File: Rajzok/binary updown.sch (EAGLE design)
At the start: 17 parts, among them Q1 TP0602N2, Q2 TP0602N2, Q3 SUP75N06-08, Q4 SUP75N06-08

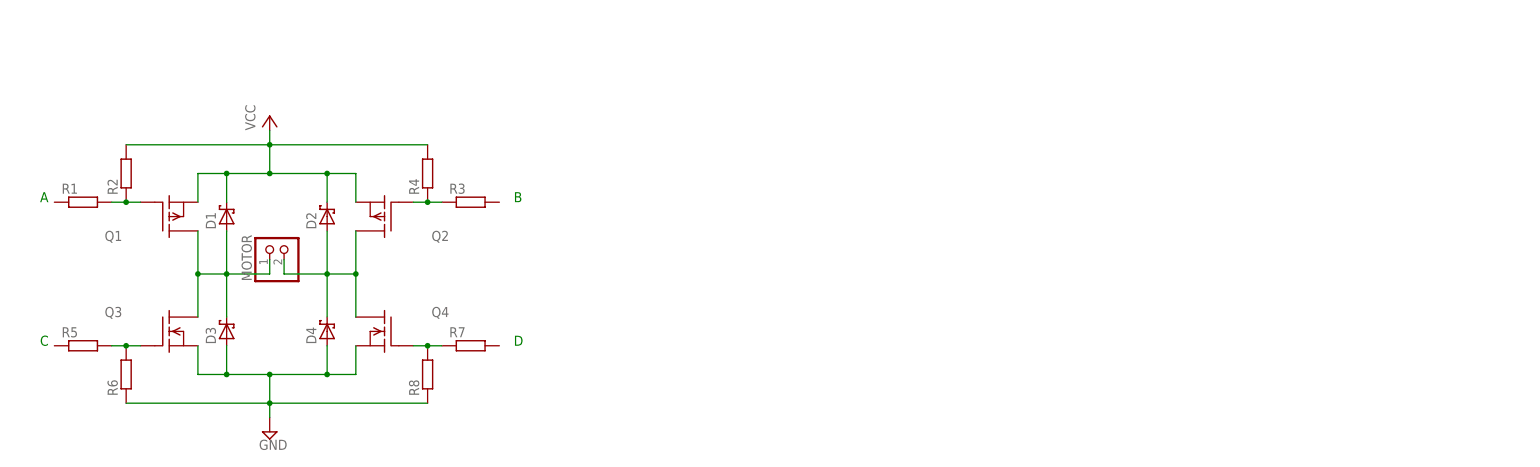
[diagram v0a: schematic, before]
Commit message: Rajzok 2017
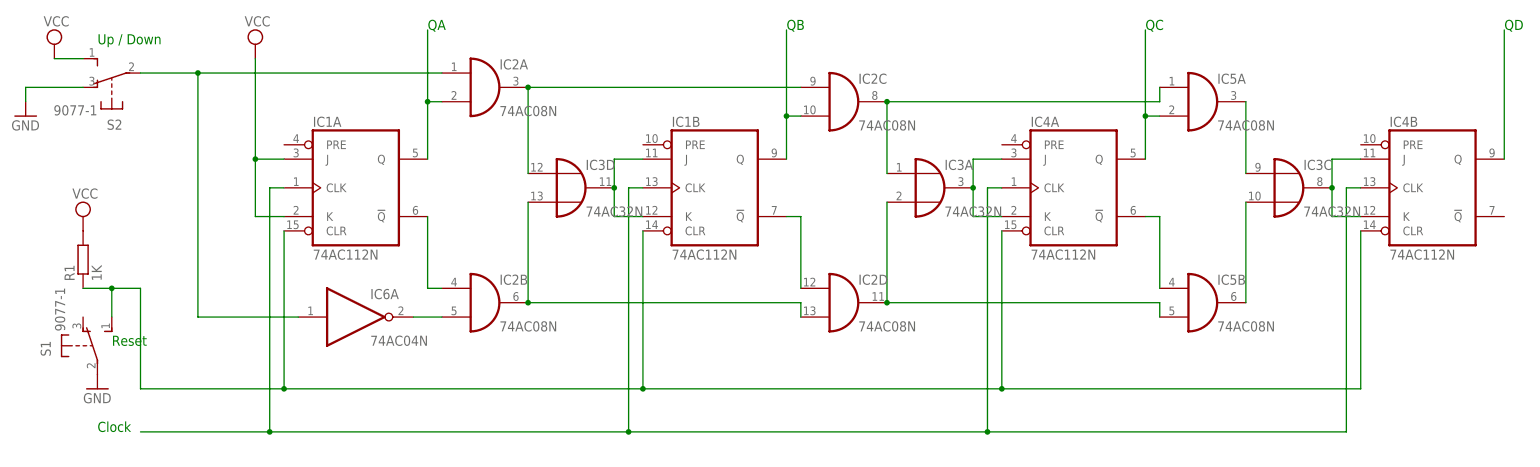
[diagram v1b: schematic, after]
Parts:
- removed D1, D2, D3, D4: 1N6267A, diode:1N6267A
- removed MOTOR: (no value), pinhead:PINHD-1X2
- removed Q1, Q2: TP0602N2, transistor-fet:TP0602N2
- removed Q3, Q4: SUP75N06-08, transistor-fet:SUP75N06-08
- removed R2, R3, R4, R5, R6, R7, R8: (no value), rcl:R-EU_0204/7
- added IC1, IC4: 74AC112N, 74xx-eu:74AC112N
- added IC2, IC5: 74AC08N, 74xx-eu:74AC08N
- added IC3: 74AC32N, 74xx-eu:74AC32N
- added IC6: 74AC04N, 74xx-eu:74AC04N
- added S1, S2: 9077-1, switch-misc:9077-1
- R1: value (none) -> 1K
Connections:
- new net N$10: IC1B.!Q, IC2D.I0
- new net N$11: IC1A.Q, IC2A.I1
- new net N$12: IC1B.Q, IC2C.I1
- new net N$13: IC4A.Q, IC5A.I1
- new net N$14: IC4A.!Q, IC5B.I0
- new net N$15: IC2A.I0, IC6A.I, S2.P
- new net N$16: IC4B.Q
- new net N$17: IC1A.CLK, IC1B.CLK, IC4A.CLK, IC4B.CLK
- new net N$18: IC1A.!Q, IC2B.I0
- new net N$19: IC2B.I1, IC6A.O
- new net N$20: IC1A.CLR, IC1B.CLR, IC4A.CLR, IC4B.CLR, R1.1, S1.S
- new net N$6: IC2C.O, IC3A.I0, IC5A.I0
- new net N$7: IC2D.O, IC3A.I1, IC5B.I1
- new net N$8: IC3C.I0, IC5A.O
- net GND: now also S1.P, S2.O; no longer D3.A, D4.A, Q3.S, Q4.S, R6.1, R8.1
- net N$1: now also IC1B.J, IC1B.K, IC3D.O; no longer Q1.G, R1.2, R2.1
- net N$2: now also IC3A.O, IC4A.J, IC4A.K; no longer D2.A, D4.C, MOTOR.2, Q2.D, Q4.D
- net N$3: now also IC3C.O, IC4B.J, IC4B.K; no longer Q2.G, R3.1, R4.1
- net N$4: now also IC2A.O, IC2C.I0, IC3D.I0; no longer Q3.G, R5.2, R6.2
- net N$5: now also IC2B.O, IC2D.I1, IC3D.I1; no longer Q4.G, R7.1, R8.2
- net N$9: now also IC3C.I1, IC5B.O; no longer D1.A, D3.C, MOTOR.1, Q1.D, Q3.D
- net VCC: now also IC1A.J, IC1A.K, R1.2, S2.S; no longer D1.C, D2.C, Q1.S, Q2.S, R2.2, R4.2
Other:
- note added: "Clock"
- note added: "QA"
- note added: "QB"
- note added: "QC"
- note added: "QD"
- note added: "Reset"
- note added: "Up / Down"
- note removed: "A"
- note removed: "B"
- note removed: "C"
- note removed: "D"
- moved on the sheet: R1
